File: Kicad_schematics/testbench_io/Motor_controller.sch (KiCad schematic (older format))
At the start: 9 parts, among them J701 DB37_Female_MountingHoles, SW701 SW_SPST, SW702 SW_SPST, SW703 SW_SPST, SW704 SW_DIP_x08

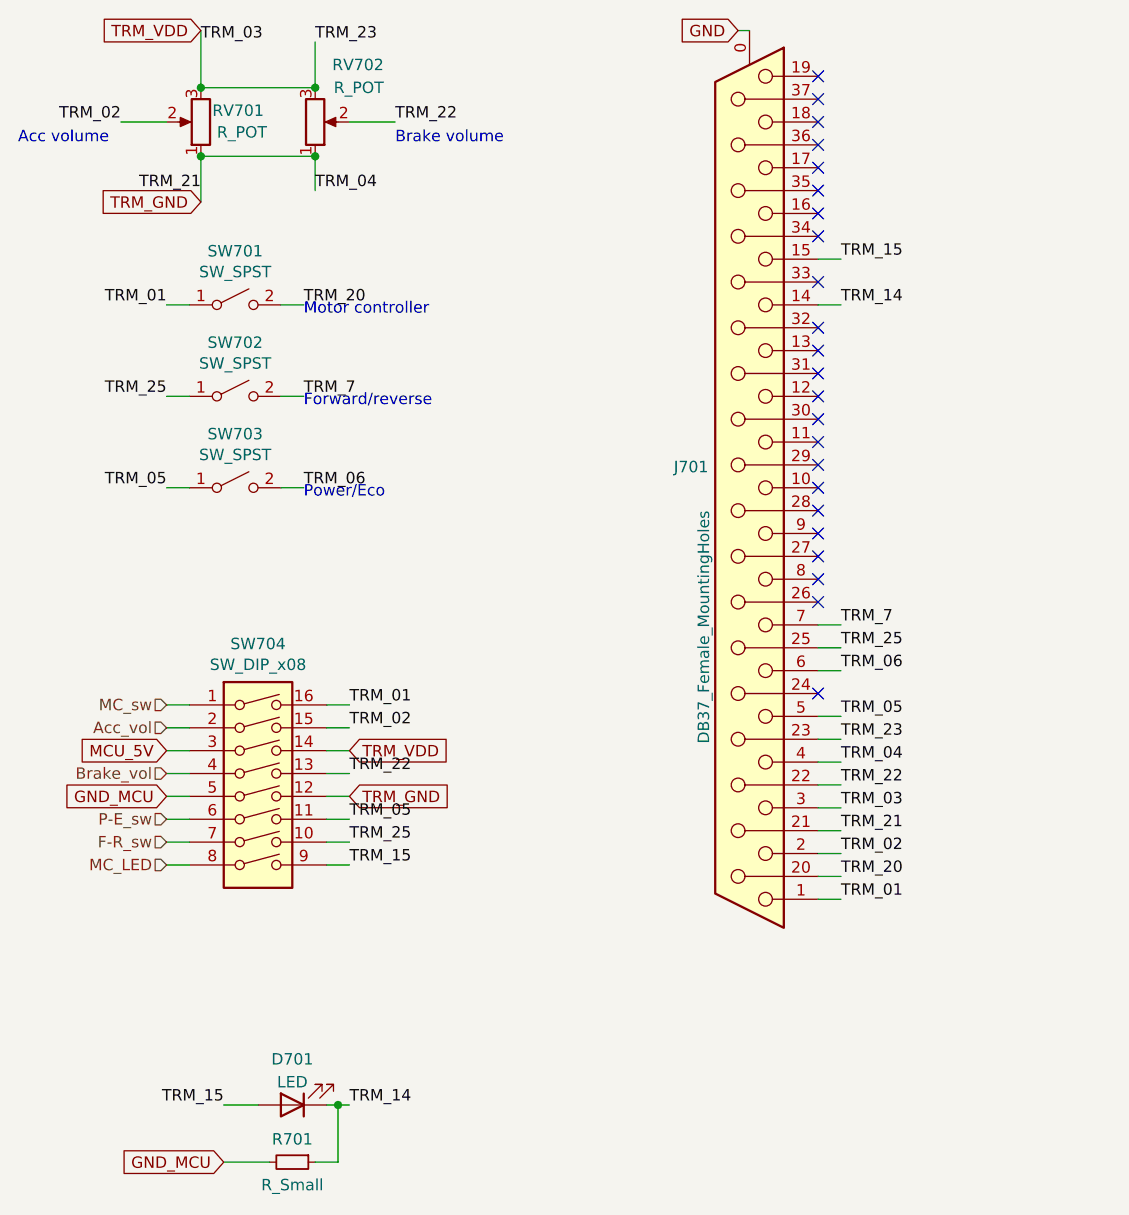
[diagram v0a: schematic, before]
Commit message: fixes
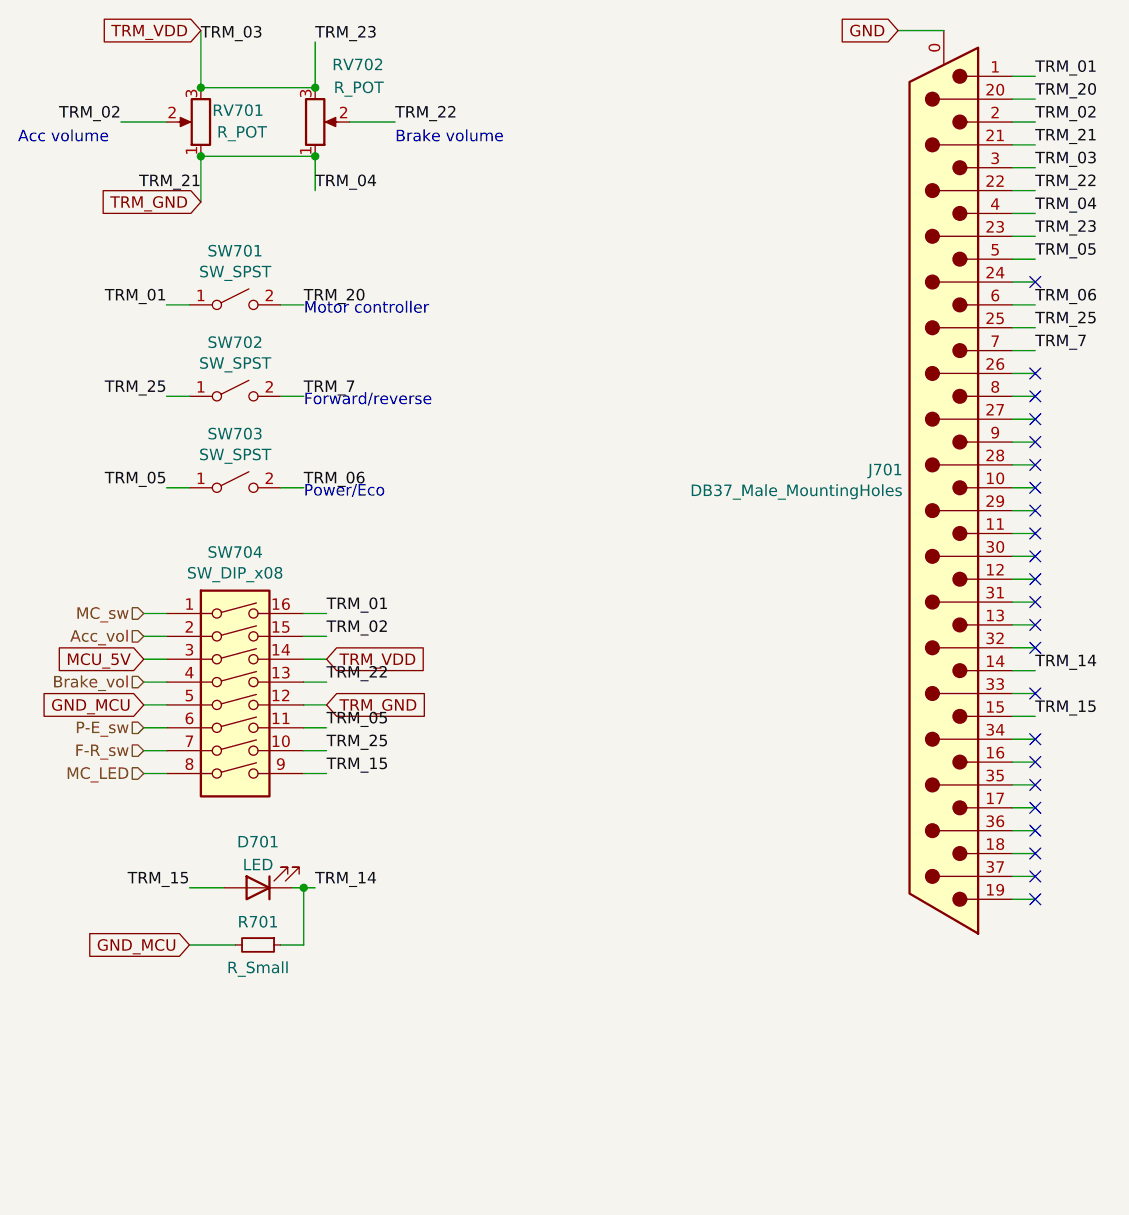
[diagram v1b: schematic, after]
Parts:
- removed J701: DB37_Female_MountingHoles, Connector_Dsub:DSUB-37_Female_Horizontal_P2.77x2.84mm_EdgePinOffset7.70mm_Housed_MountingHolesOffset9.12mm, symbol Connector:DB37_Female_MountingHoles
- added J701: DB37_Male_MountingHoles, Solar_team:Wurth_Dsub_37_angled_male_8.08mm, symbol Connector:DB37_Male_MountingHoles
- SW701, SW702, SW703: footprint Solar_team:RND-Slide-Switch -> Solar_team:MFP120
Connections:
- net GND: now also J701.0 (PAD)
- net TRM_01: now also J701.1
- net TRM_02: now also J701.2
- net TRM_05: now also J701.5
- net TRM_06: now also J701.6
- net TRM_14: now also J701.14
- net TRM_15: now also J701.15
- net TRM_20: now also J701.20
- net TRM_22: now also J701.22
- net TRM_25: now also J701.25
- net TRM_7: now also J701.7
- net TRM_GND: now also J701.21, J701.4
- net TRM_VDD: now also J701.23, J701.3
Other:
- moved on the sheet: D701, R701, SW704
